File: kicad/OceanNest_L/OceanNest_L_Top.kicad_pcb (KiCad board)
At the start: 2 copper layers, 126.4 x 94.7 mm, 18 parts, among them SW21 SW_Push, SW22 SW_Push, SW23 SW_Push, SW24 SW_Push, SW25 SW_Push, SW26 SW_Push, SW27 SW_Push, SW28 SW_Push, SW29 SW_Push, SW30 SW_Push, SW31 SW_Push, SW32 SW_Push, SW33 SW_Push, SW34 SW_Push

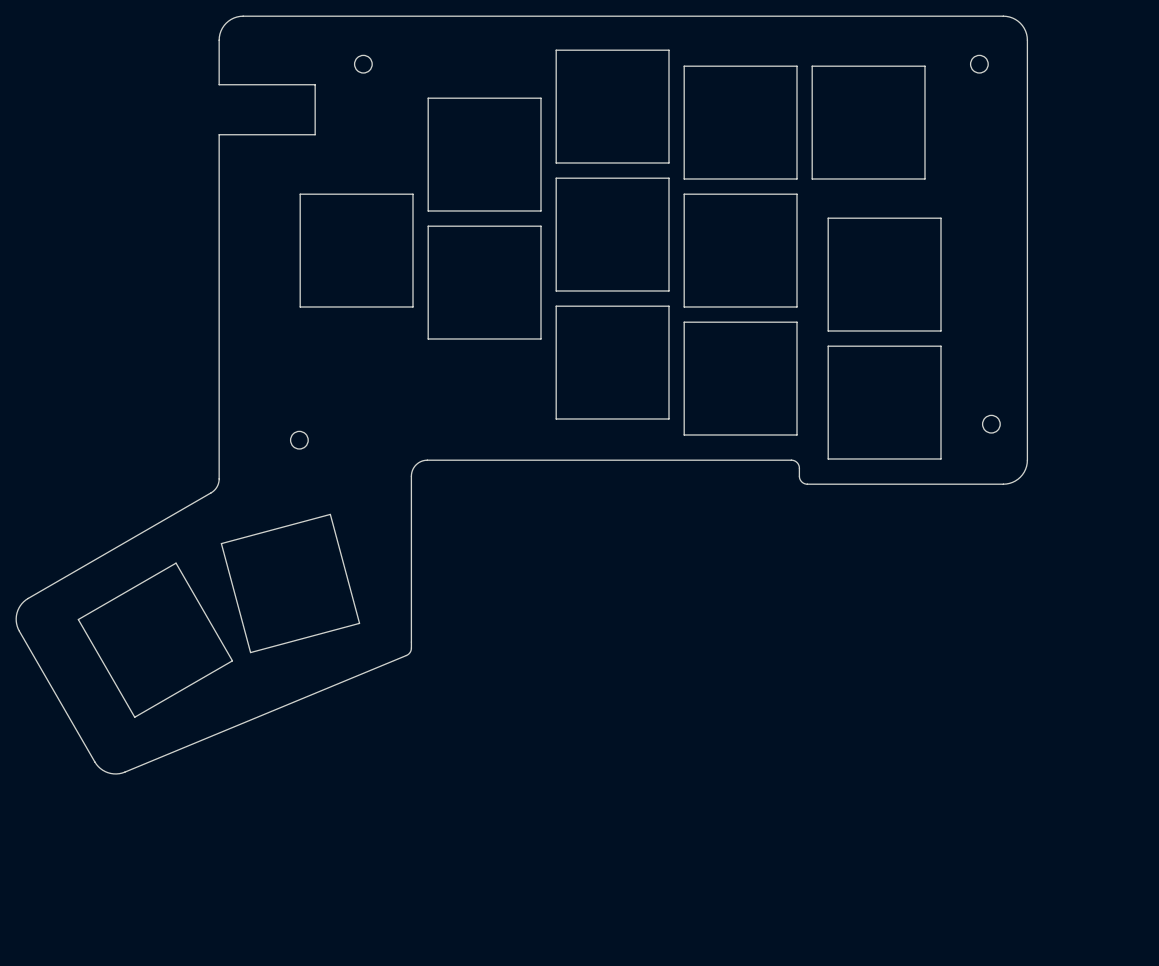
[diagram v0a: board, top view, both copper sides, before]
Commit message: routing
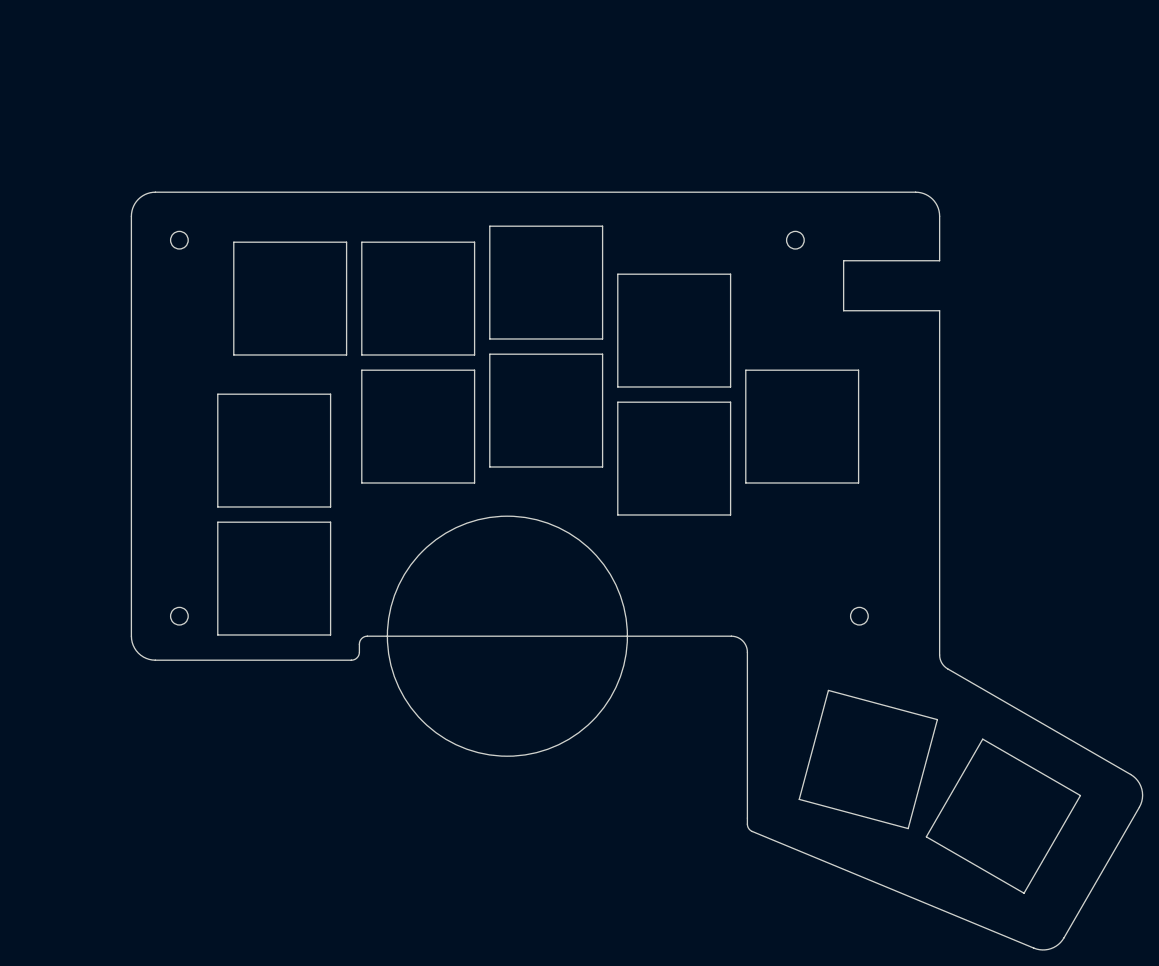
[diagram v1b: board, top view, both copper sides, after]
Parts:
- removed SW31, SW32: SW_Push, isw-kbd:SW_Hole_CherryMX_16mm
- SW21, SW22, SW23, SW24, SW25, SW26, SW27, SW28, SW29, SW30, SW33, SW34, hole1, hole2 (x3): moved to B.Cu
- moved SW33 108.3 mm to (203.0, 142.0), turned to 150 degrees
- moved hole2 104.3 mm to (100.0, 117.0), turned to 180 degrees
- moved hole2 102.4 mm to (100.0, 70.0), turned to 180 degrees
- moved SW29 79.4 mm to (111.8, 96.3), turned to 180 degrees
- moved SW30 79.4 mm to (111.8, 112.3), turned to 180 degrees
- moved SW24 75.6 mm to (113.8, 77.3), turned to 180 degrees
- moved SW34 75.5 mm to (186.1, 134.9), turned to 165 degrees
- moved hole1 73.4 mm to (185.0, 117.0), turned to 180 degrees
- moved SW25 59.9 mm to (177.8, 93.3), turned to 180 degrees
- moved hole2 58.3 mm to (177.0, 70.0), turned to 180 degrees
- moved SW28 45.9 mm to (129.8, 93.3), turned to 180 degrees
- moved SW23 45.9 mm to (129.8, 77.3), turned to 180 degrees
- moved SW26 32.3 mm to (161.8, 97.3), turned to 180 degrees
- moved SW21 32.3 mm to (161.8, 81.3), turned to 180 degrees
- moved SW27 23.5 mm to (145.8, 91.3), turned to 180 degrees
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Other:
- outline, holes or cut-outs redrawn
